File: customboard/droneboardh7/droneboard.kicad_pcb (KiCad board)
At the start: 4 copper layers, 38 x 38 mm, 62 parts, among them J1 Conn_01x04, J10 Conn_01x03_Pin, J2 Conn_01x04, J3 Conn_01x05_Pin, J4 Conn_01x02_Pin, J5 USB_C_Receptacle_USB2.0_16P, J6 Conn_01x04, SW1 SW_Push, SW2 SW_Push, U1 AP62300Z6, U2 STM32H723VGTx, U4 ICM-42688-P, U5 SPX3819M5-L-3-3, U6 SPX3819M5-L-3-3, Y2 CSTNE20M0V53Z000R0

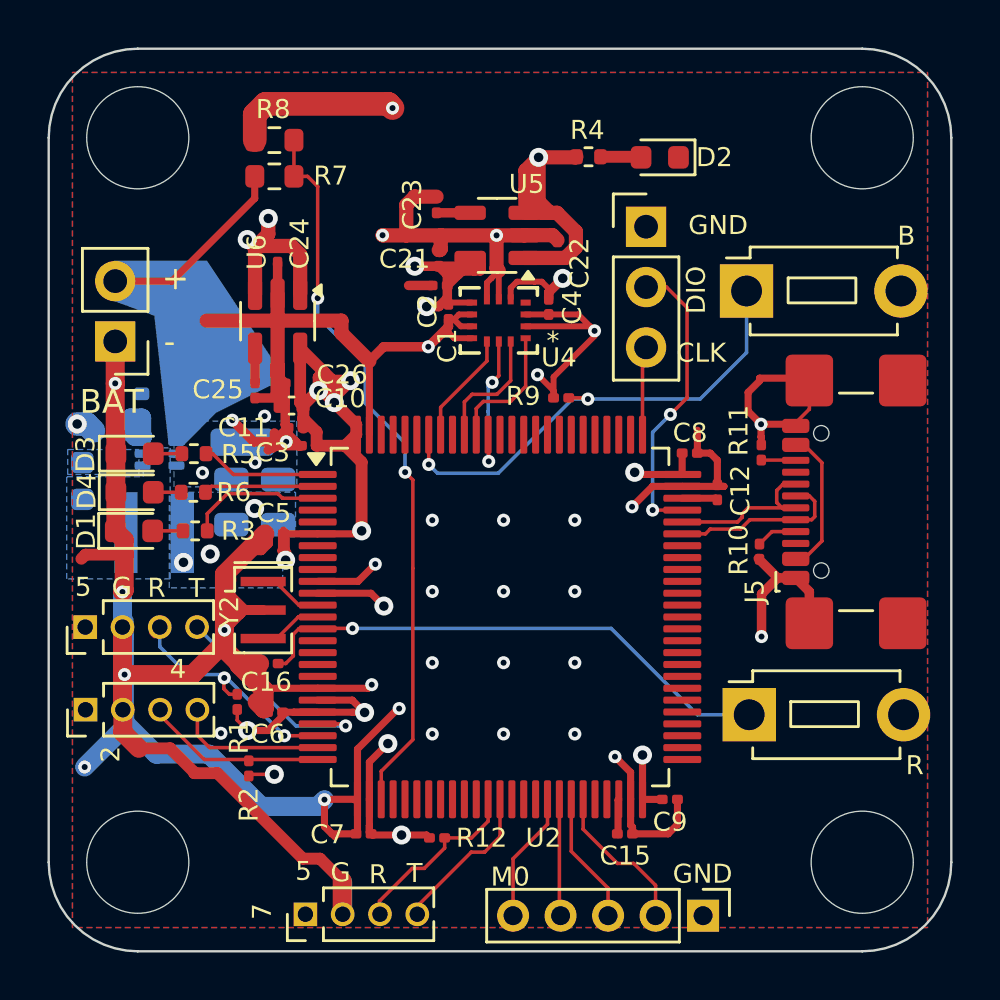
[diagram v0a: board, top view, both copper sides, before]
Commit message: stuff
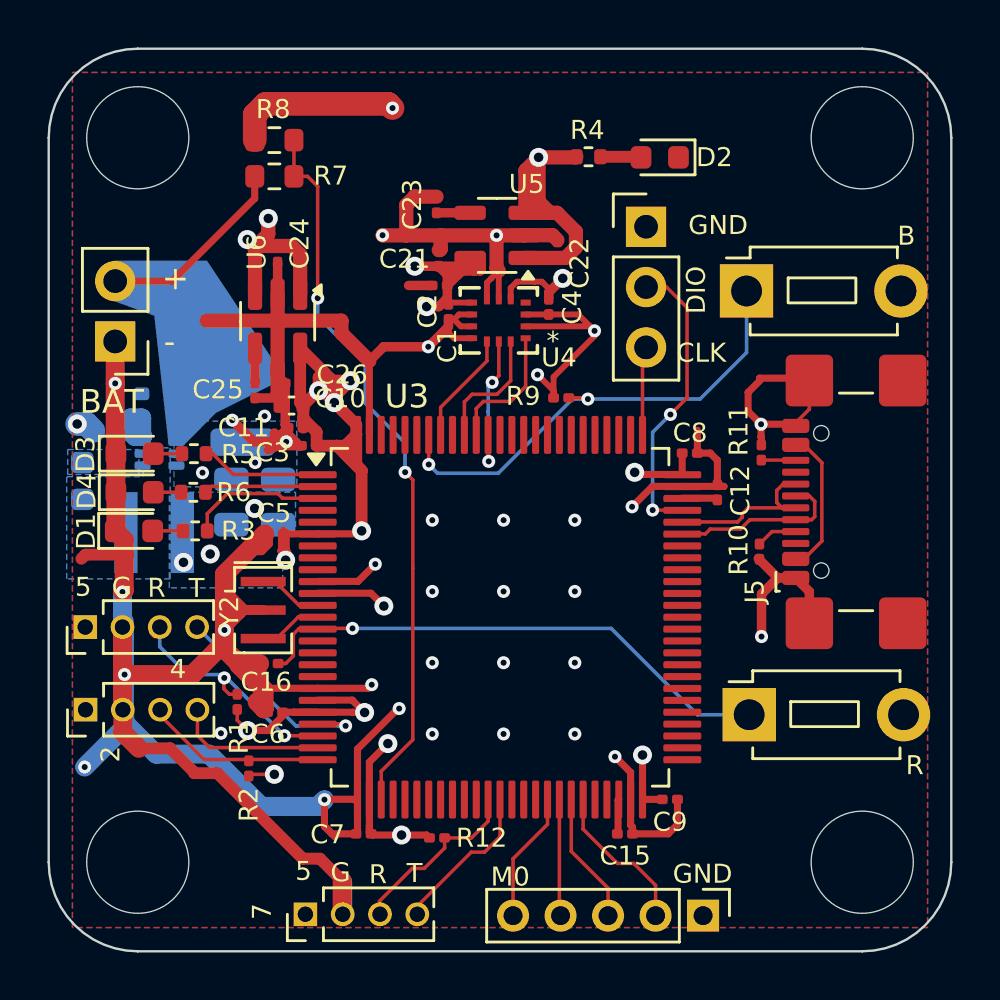
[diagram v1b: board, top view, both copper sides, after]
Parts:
- removed U2: STM32H723VGTx, Package_QFP:LQFP-100_14x14mm_P0.5mm
- added U3: STM32H743VITx, Package_QFP:LQFP-100_14x14mm_P0.5mm, F.Cu at (69.0, 105.9)
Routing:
- net /VMCU: track 51.6 -> 54.6 mm
